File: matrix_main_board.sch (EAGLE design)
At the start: 129 parts, among them IC1 MKE02_44PIN, IC2 24AA01SM, IC3 74HC595D, IC4 74HC595D, IC5 74HC595D, IC6 74HC595D, IC7 NPIC6C596, IC8 NPIC6C596

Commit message: work in prog
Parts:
- removed IC1: MKE02_44PIN, jason_eagle6:MKE02_44PIN
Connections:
- net +5V: no longer IC1.VDD, IC1.VDD1, IC1.VDDA/REFH
- net AUXIN: no longer IC1.PTC7
- net AUXOUT: no longer IC1.PTA7
- net D_ACK: no longer IC1.PTB2
- net D_ADT: no longer IC1.PTB3
- net D_ARK: no longer IC1.PTC0
- net D_ENA: no longer IC1.PTA1
- net D_KCK: no longer IC1.PTC1
- net D_KDT: no longer IC1.PTD5
- net ENC1: no longer IC1.PTD1
- net ENC2: no longer IC1.PTD0
- net GATE1: no longer IC1.PTD2
- net GATE2: no longer IC1.PTD3
- net GATE3: no longer IC1.PTD4
- net GATE4: no longer IC1.PTA6
- net GND: no longer IC1.VSS, IC1.VSS1, IC1.VSSA/VSS
- net I2C0SCL: no longer IC1.PTA3
- net I2C0SDA: no longer IC1.PTA2
- net I2C1SCL: no longer IC1.PTE1
- net I2C1SDA: no longer IC1.PTE0
- net KEY_READ1: no longer IC1.PTC6
- net KEY_READ2: no longer IC1.PTB4
- net LED1: no longer IC1.PTB5
- net LED2: no longer IC1.PTC3
- net LED3: no longer IC1.PTC2
- net MIDIRX: no longer IC1.PTB0
- net MIDITX: no longer IC1.PTB1
- net OFF_SW: no longer IC1.PTE7
- net PWR_CTRL: no longer IC1.PTE2
- net SYNCIN: no longer IC1.PTA0
- net SYNCOUT: no longer IC1.PTC5
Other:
- note added: "Version 4 - 30 JUL 22 - J Hotchkiss / Sixty Four Pixels"
- note removed: "Version 3 - 26 NOV 19 - J Hotchkiss / Sixty Four Pixels"
- moved on the sheet: C1, C11, C2, C4, GD4, PD6, PD7, PH2, R3, R4, R5, R6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

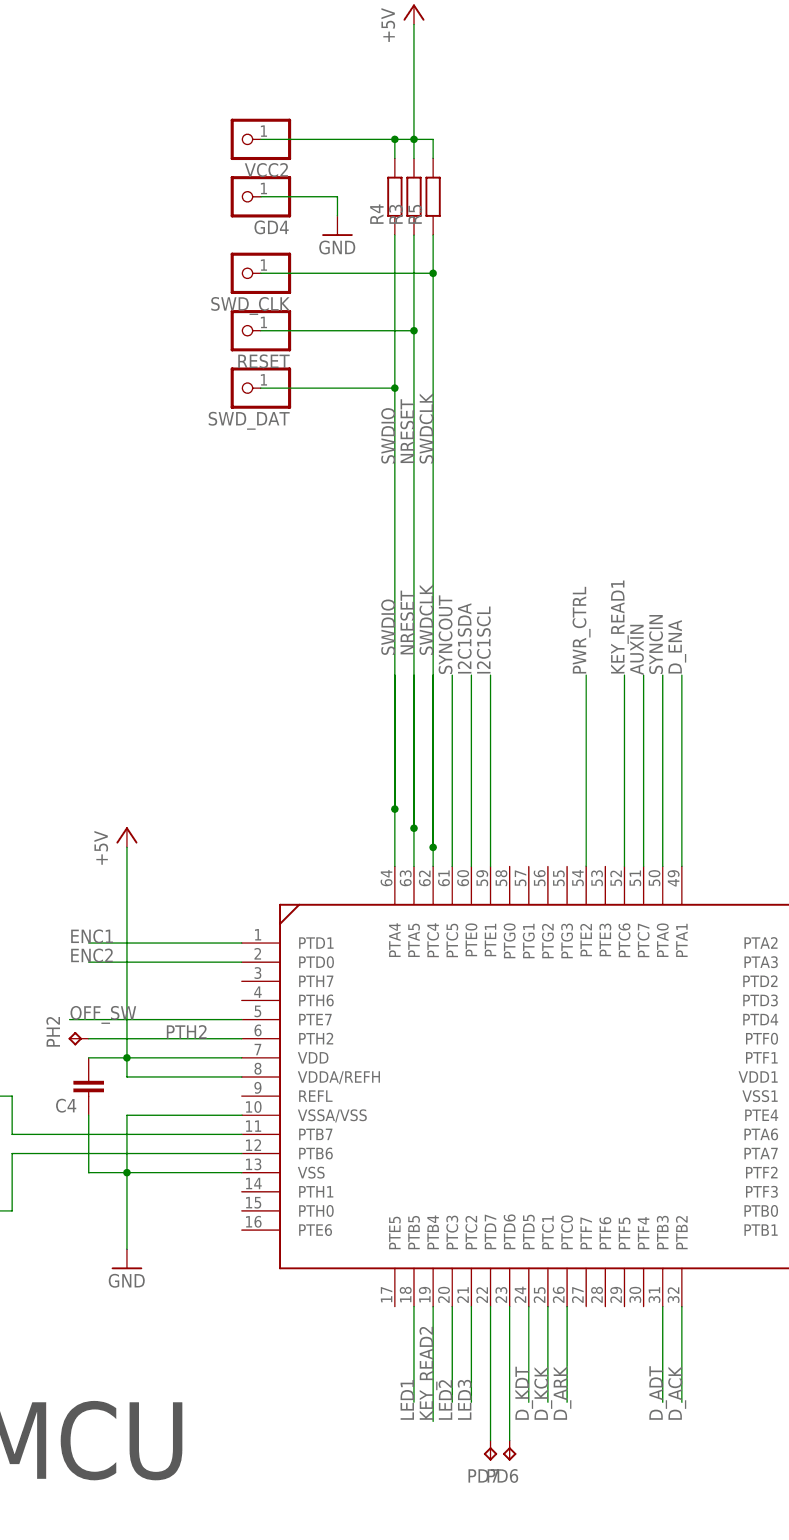
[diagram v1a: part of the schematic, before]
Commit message: 64pin
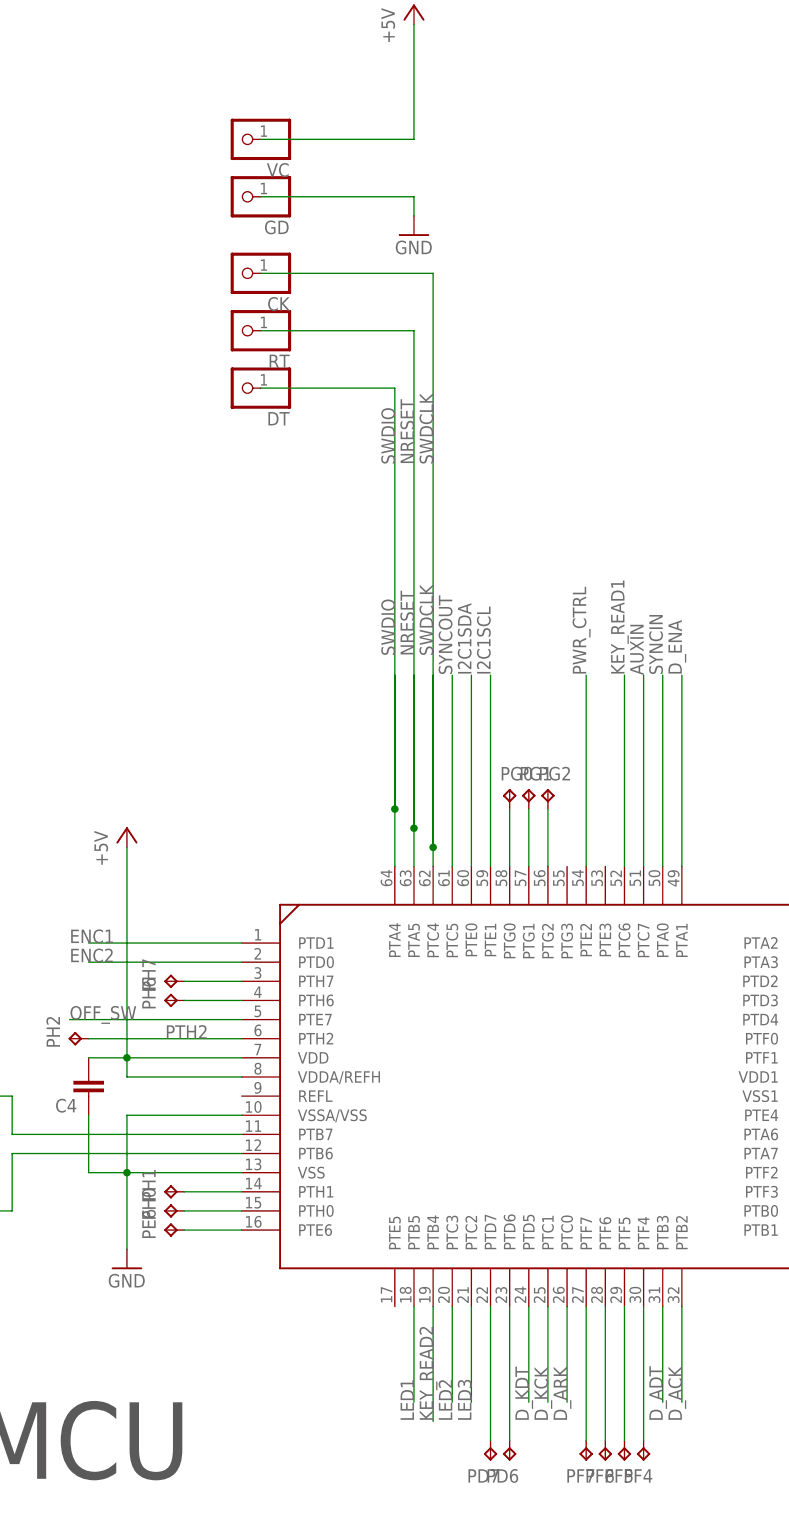
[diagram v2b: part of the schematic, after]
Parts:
- removed R3, R4, R5: (no value), rcl:R-EU_R0805
- added PE6, PF4, PF5, PF6, PF7, PG0, PG1, PG2, PH0, PH1, PH6, PH7: TPTP17R, testpad:TPTP17R
- renumbered GD4 to GD, RESET to RT, SWD_CLK to CK, SWD_DAT to DT, U$1 to IC1, VCC2 to VC
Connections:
- new net N$15: IC1.PTF7, PF7.TP
- new net N$25: IC1.PTF6, PF6.TP
- new net N$26: IC1.PTF5, PF5.TP
- new net N$27: IC1.PTF4, PF4.TP
- new net N$36: IC1.PTH1, PH1.TP
- new net N$37: IC1.PTH0, PH0.TP
- new net N$38: IC1.PTE6, PE6.TP
- new net N$41: IC1.PTH6, PH6.TP
- new net N$43: IC1.PTG1, PG1.TP
- new net PG0: IC1.PTG0, PG0.TP
- new net PTG2: IC1.PTG2, PG2.TP
- new net PTH7: IC1.PTH7, PH7.TP
- net +5V: no longer R3.2, R4.2, R5.2
- net NRESET: no longer R3.1
- net SWDCLK: no longer R5.1
- net SWDIO: no longer R4.1
